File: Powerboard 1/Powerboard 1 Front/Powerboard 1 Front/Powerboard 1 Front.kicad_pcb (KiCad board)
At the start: 2 copper layers, 40 x 128.5 mm, 0 parts

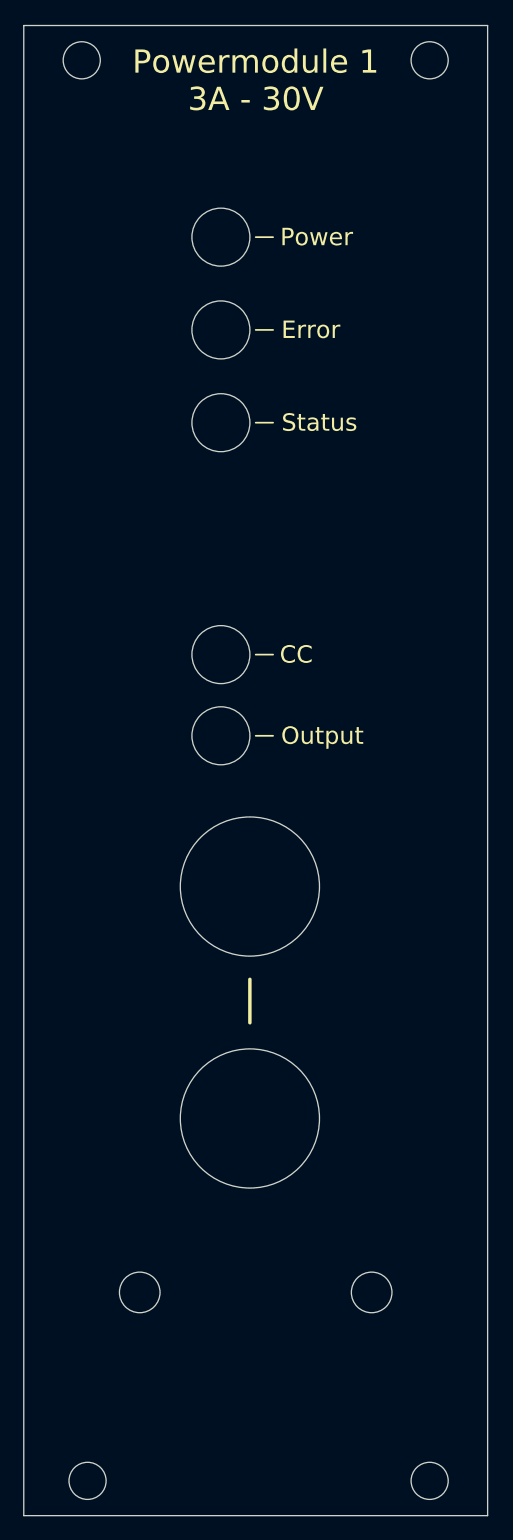
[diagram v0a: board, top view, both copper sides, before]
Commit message: Rev 3 Pcb's
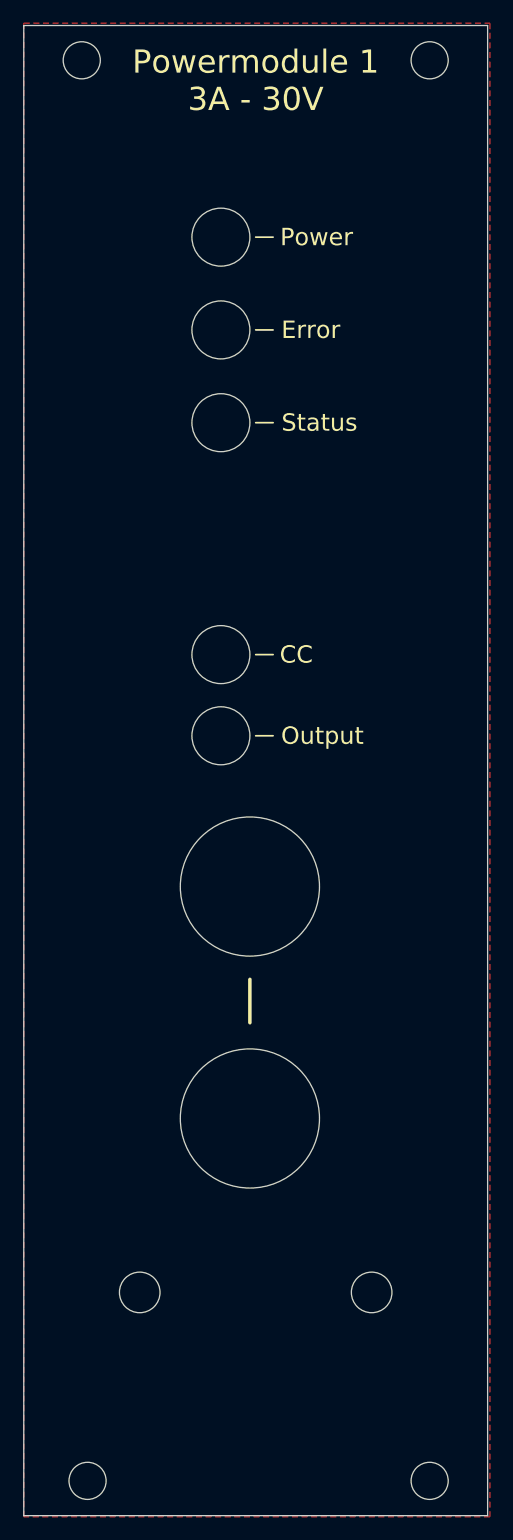
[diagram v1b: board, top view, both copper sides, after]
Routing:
- added copper zone on F.Cu, net (none)
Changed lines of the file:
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@@
       (drillshape 0)
       (scaleselection 1)
-      (outputdirectory "")
+      (outputdirectory "Gerber/")
     )
   )
@@
     (effects (font (size 1.5 1.5) (thickness 0.15)))
   )
+  (zone (net 0) (net_name "") (layer "F.Cu") (hatch edge 0.508)
+    (connect_pads (clearance 0.508))
+    (min_thickness 0.254) (filled_areas_thickness no)
+    (fill yes (thermal_gap 0.508) (thermal_bridge_width 0.508) (smoothing fillet) (radius 1))
+    (polygon
+      (pts
+        (xy 60.2 148.6)
+        (xy 20 148.6)
+        (xy 20 19.8)
+        (xy 60.2 19.8)
+      )
+    )
+  )
 )
